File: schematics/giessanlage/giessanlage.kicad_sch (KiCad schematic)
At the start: 17 parts, among them P1 Pumpe, P2 Pumpe, Q1 IRLZ34N, Q2 IRLZ34N, SW1 P1_Manuell_On, SW2 P1_Manuell_On, SW3 Manuell_Off, U1 ESP32-C6-DevKitC-1

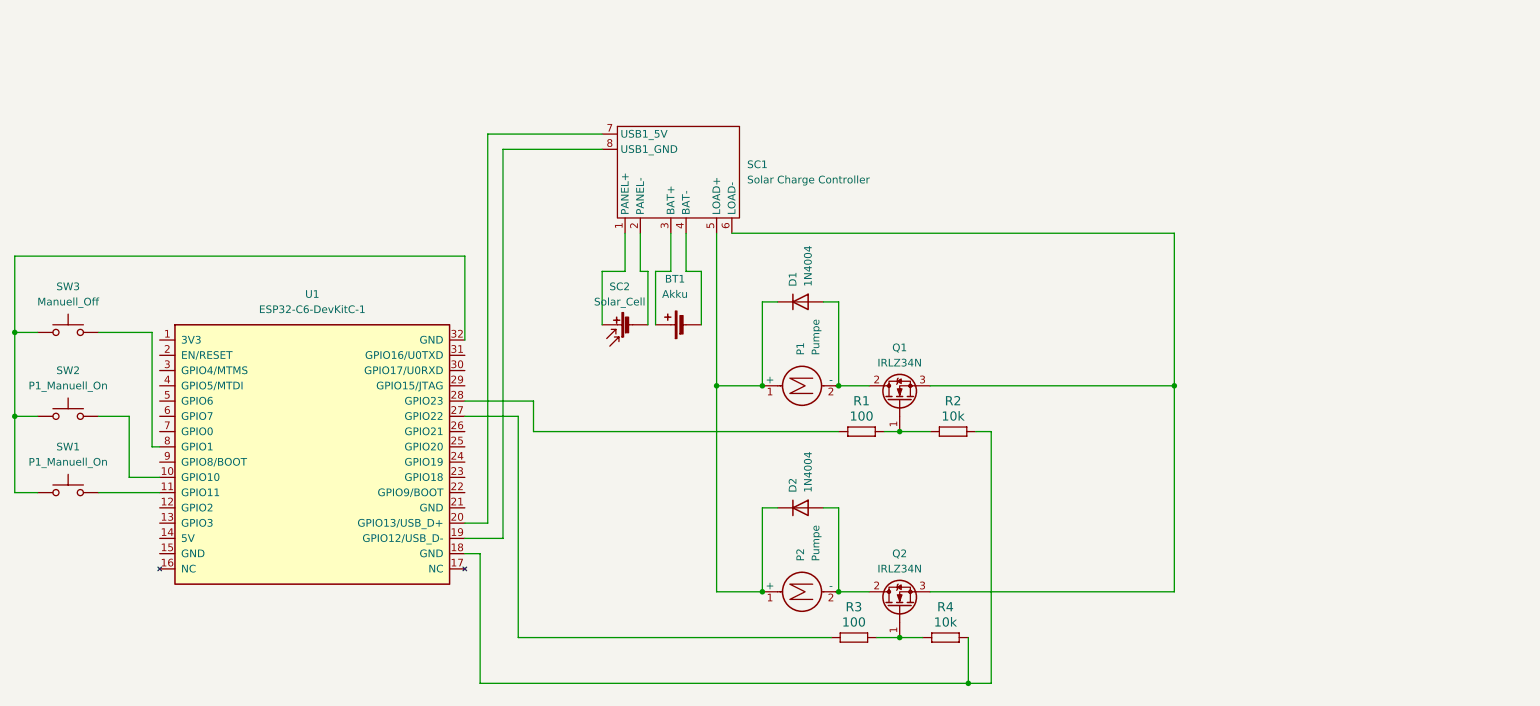
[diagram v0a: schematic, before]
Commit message: feat: schematics and doc update
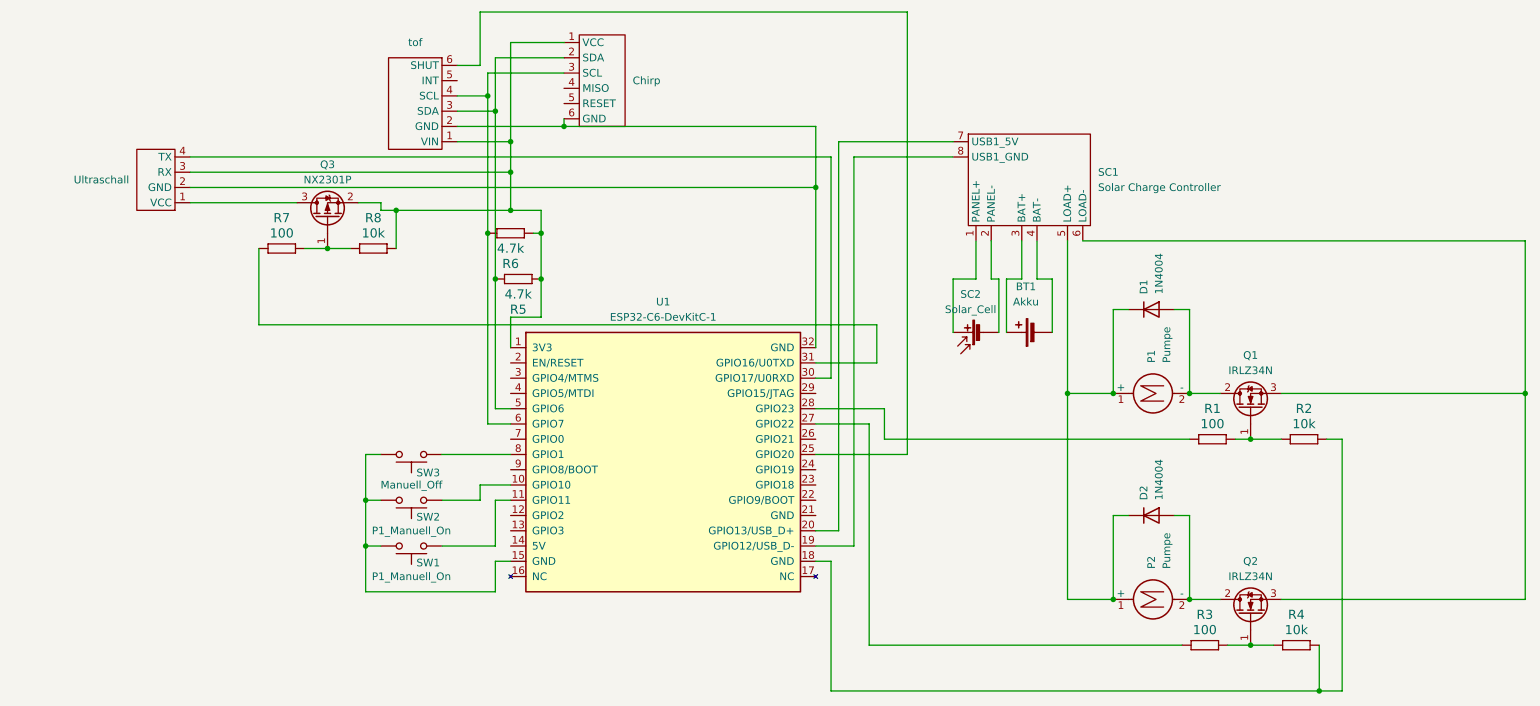
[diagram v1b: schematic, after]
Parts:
- added Chirp: (no value), symbol 01_own:Chirp
- added Q3: NX2301P, Package_TO_SOT_SMD:SOT-23, symbol Transistor_FET:IRLML6402
- added R5, R6: 4.7k, symbol CERN:Resistor
- added R7: 100, symbol CERN:Resistor
- added R8: 10k, symbol CERN:Resistor
- added Ultraschall: (no value), symbol 01_own:Ultraschall
- added tof: (no value), symbol 01_own:Tof
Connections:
- net at SW1.1, SW2.1, SW3.1: now also U1.15 (GND); no longer U1.32 (GND)
- net at U1.1 (3V3): now also Chirp.1 (VCC), Q3.2 (S), R5.1, R6.1, R8.2, Ultraschall.3 (RX), tof.1 (VIN)
- net at U1.25 (GPIO20): now also tof.6 (SHUT)
- net at U1.30 (GPIO17/U0RXD): now also Ultraschall.4 (TX)
- net at U1.31 (GPIO16/U0TXD): now also R7.1
- net at U1.5 (GPIO6): now also Chirp.2 (SDA), R5.2, tof.3 (SDA)
- net at U1.6 (GPIO7): now also Chirp.3 (SCL), R6.2, tof.4 (SCL)
- new net: Q3.1 (G), R7.2, R8.1
- new net: Chirp.6 (GND), U1.32 (GND), Ultraschall.2 (GND), tof.2 (GND)
- new net: Q3.3 (D), Ultraschall.1 (VCC)
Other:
- moved on the sheet: BT1, D1, D2, P1, P2, Q1, Q2, R1, R2, R3, R4, SC1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
